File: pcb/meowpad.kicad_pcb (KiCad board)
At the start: 2 copper layers, 110 x 65.5 mm, 16 parts, among them J1 OLED_DISPLAY, SW1 SW_Push_45deg, SW2 SW_Push_45deg, SW3 SW_Push_45deg, SW4 SW_Push_45deg, SW6 SW_Push_45deg, U2 XIAO-RP2040-DIP

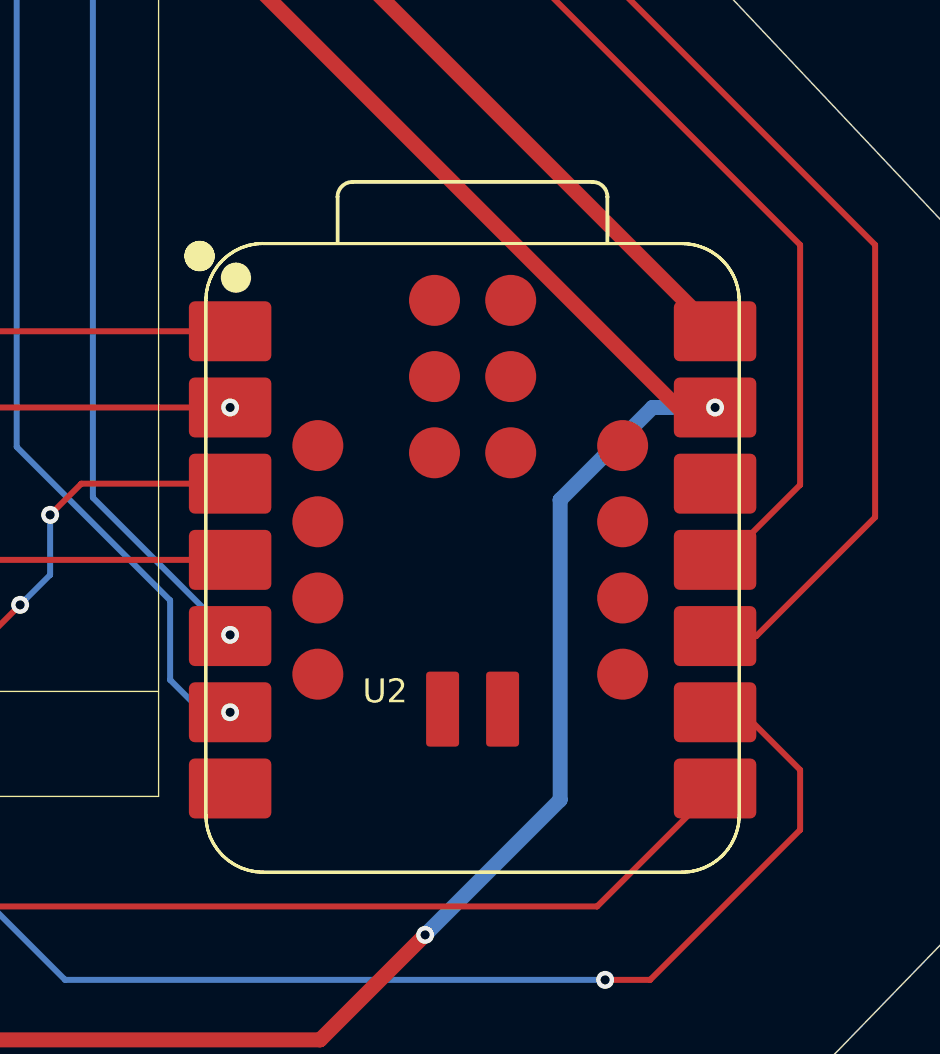
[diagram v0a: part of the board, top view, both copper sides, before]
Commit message: bill of materials
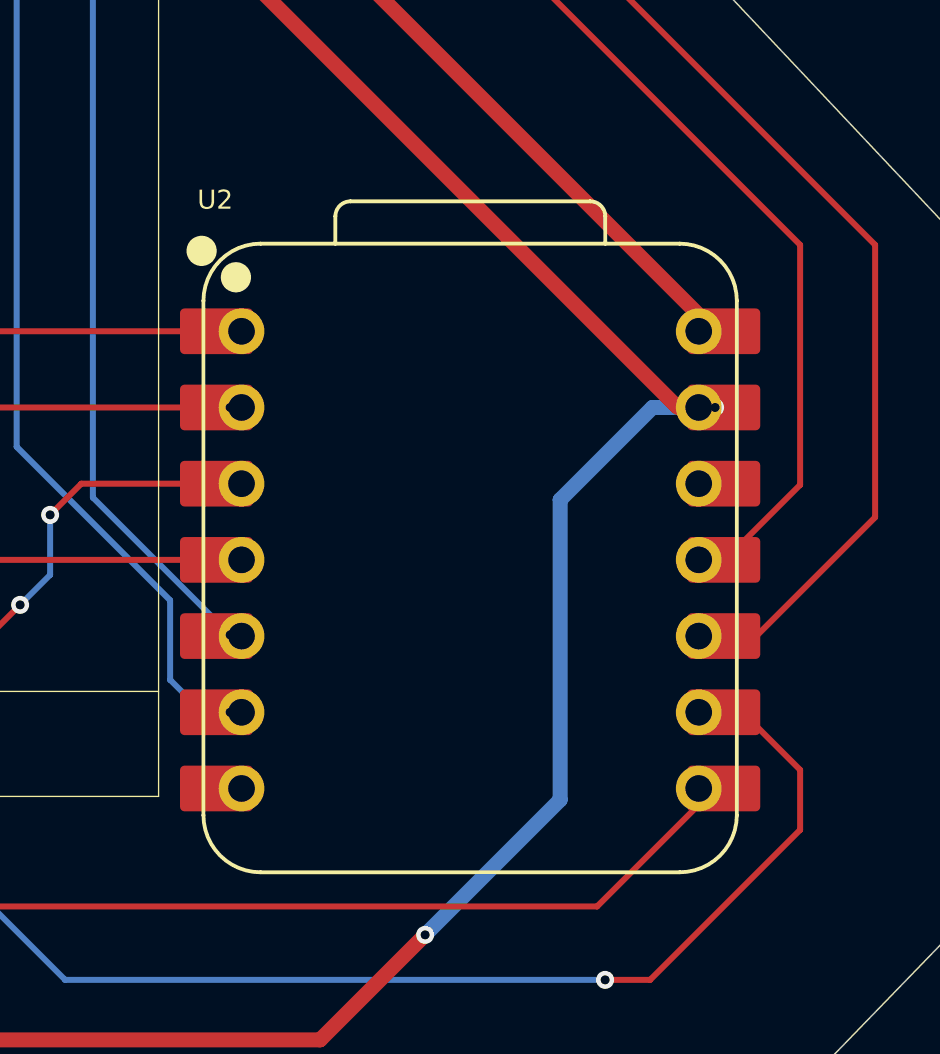
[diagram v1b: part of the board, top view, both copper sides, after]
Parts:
- U2: footprint Seeed Studio XIAO Series Library:XIAO-RA4M1-SMD -> Seeed Studio XIAO Series Library:XIAO-RP2040-DIP
